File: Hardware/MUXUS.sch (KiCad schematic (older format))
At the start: 3 parts

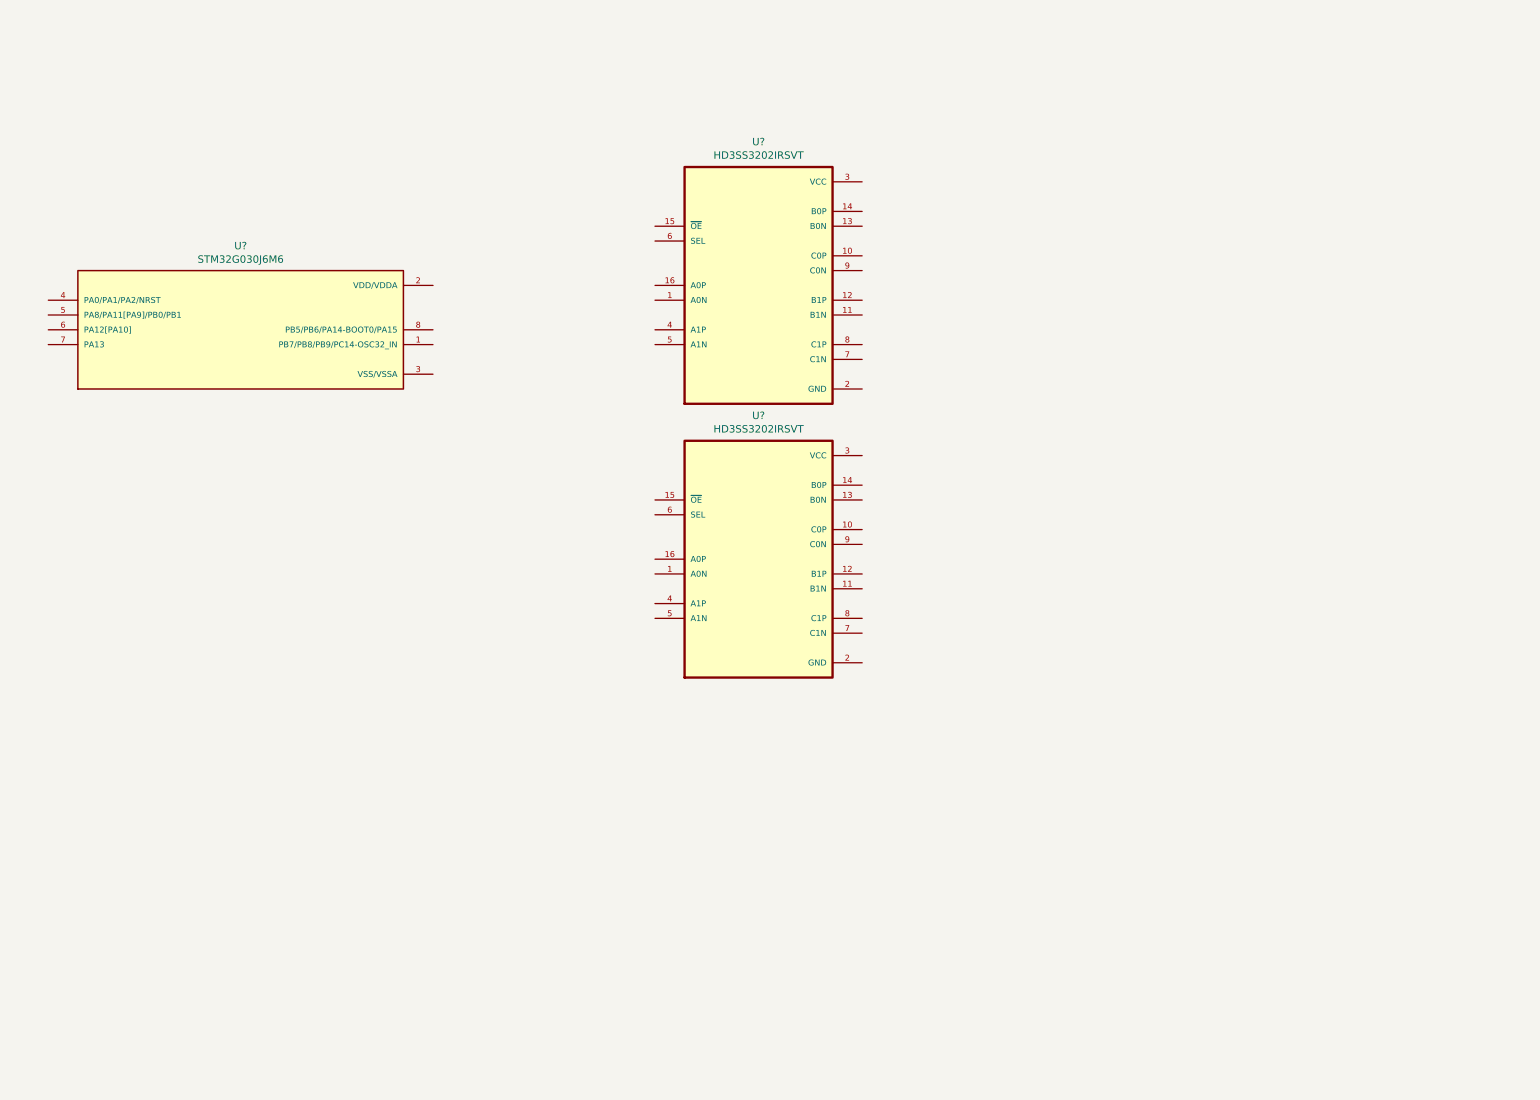
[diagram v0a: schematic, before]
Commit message: Checkpoint
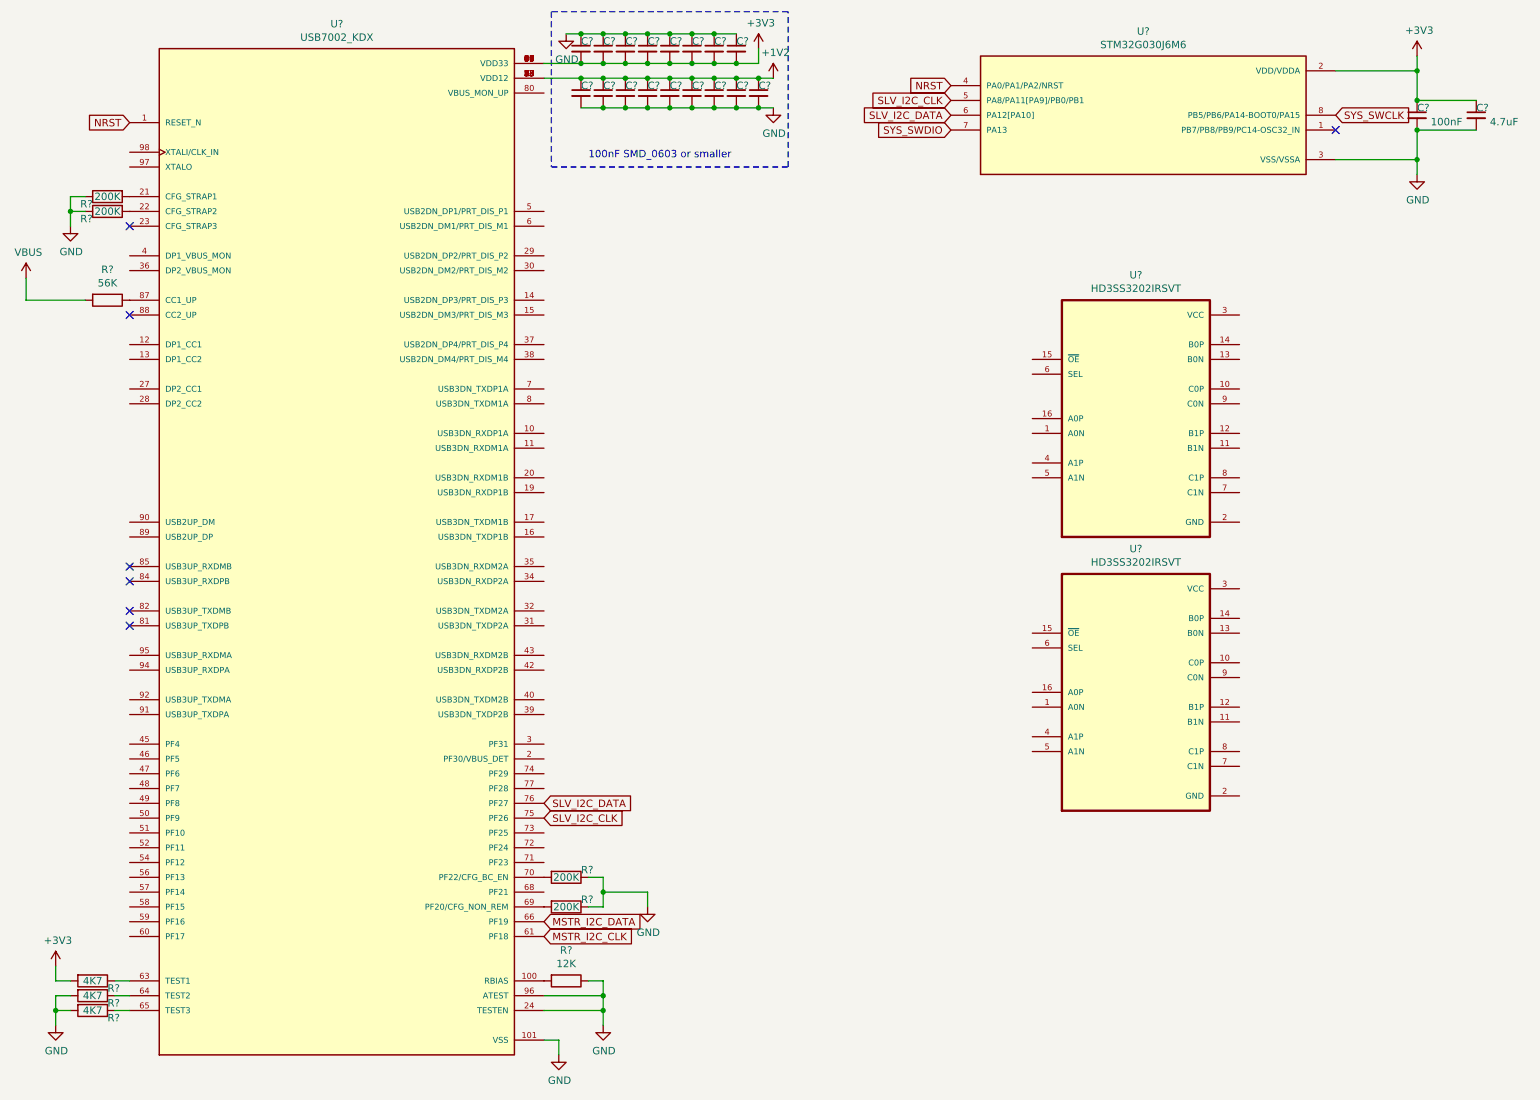
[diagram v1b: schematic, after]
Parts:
- added C? (x18): 100nF, symbol Device:C_Small
- added C?: 4.7uF, symbol Device:C_Small
- added R?: 12K, symbol Device:R
- added R? (x3): 4K7, symbol Device:R
- added R? (x4): 200K, symbol Device:R
- added R?: 56K, symbol Device:R
- added U?: USB7002_KDX, QFN40P1200X1200X90-101N, symbol USB7002_KDX:USB7002_KDX
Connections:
- net +3V3: now reaches U?.2 (VDD/VDDA)
- net +3V3: now also C?.1, C?.1, C?.2, C?.2, C?.2, C?.2, C?.2, C?.2, C?.2, C?.2, R?.2, U?.26 (VDD33), U?.44 (VDD33), U?.53 (VDD33), U?.62 (VDD33), U?.67 (VDD33), U?.79 (VDD33), U?.86 (VDD33), U?.99 (VDD33)
- net GND: now reaches U?.3 (VSS/VSSA)
- net GND: now also C?.1, C?.1, C?.1, C?.1, C?.1, C?.1, C?.1, C?.1, C?.2, C?.2, C?.2, C?.2, C?.2, C?.2, C?.2, C?.2, C?.2, C?.2, C?.2, R?.1, R?.1, R?.1, R?.1, R?.1, R?.2, R?.2, U?.101 (VSS), U?.24 (TESTEN), U?.96 (ATEST)
- net NRST: now reaches U?.4 (PA0/PA1/PA2/NRST)
- net NRST: now also U?.1 (RESET_N)
- net SLV_I2C_CLK: now reaches U?.5 (PA8/PA11[PA9]/PB0/PB1)
- net SLV_I2C_CLK: now also U?.75 (PF26)
- net SLV_I2C_DATA: now reaches U?.6 (PA12[PA10])
- net SLV_I2C_DATA: now also U?.76 (PF27)
- net SYS_SWDIO: now reaches U?.7 (PA13)
- net SYS_SWCLK: now reaches U?.8 (PB5/PB6/PA14-BOOT0/PA15)
- new net: R?.2, U?.100 (RBIAS)
- new net: R?.2, U?.21 (CFG_STRAP1)
- new net: R?.2, U?.22 (CFG_STRAP2)
- new net: R?.1, U?.63 (TEST1)
- new net: R?.1, U?.64 (TEST2)
- new net: R?.1, U?.65 (TEST3)
- new net: R?.2, U?.69 (PF20/CFG_NON_REM)
- new net: R?.2, U?.70 (PF22/CFG_BC_EN)
- new net: R?.1, U?.87 (CC1_UP)
- new net +1V2: C?.1, C?.1, C?.1, C?.1, C?.1, C?.1, C?.1, C?.1, C?.1, U?.18 (VDD12), U?.25 (VDD12), U?.33 (VDD12), U?.41 (VDD12), U?.55 (VDD12), U?.78 (VDD12), U?.83 (VDD12), U?.9 (VDD12), U?.93 (VDD12)
- new net MSTR_I2C_CLK: U?.61 (PF18)
- new net MSTR_I2C_DATA: U?.66 (PF19)
- new net VBUS: R?.2
- no-connect marks 0 -> 7
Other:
- note added: "100nF SMD_0603 or smaller"
- moved on the sheet: U?

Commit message: Checkpoint
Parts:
- removed C? (x18): 100nF, symbol Device:C_Small
- removed C?: 4.7uF, symbol Device:C_Small
- removed R?: 12K, symbol Device:R
- removed R? (x3): 4K7, symbol Device:R
- removed R? (x4): 200K, symbol Device:R
- removed R?: 56K, symbol Device:R
- removed U? (x2): HD3SS3202IRSVT, QFN40P180X260X55-16N_HD3SS3202IRSVT, symbol HD3SS3202IRSVT:HD3SS3202IRSVT
- removed U?: STM32G030J6M6, SOIC127P600X175-8N, symbol STM32G030J6M6:STM32G030J6M6
- removed U?: USB7002_KDX, QFN40P1200X1200X90-101N, symbol USB7002_KDX:USB7002_KDX
- added C? (x11): 100nF, Capacitor_SMD:C_0805_2012Metric, symbol Device:C_Small
- added C? (x5): 4.7uF, symbol Device:C_Small
- added C?: 87pF, symbol Device:C
- added C? (x14): 100nF, Capacitor_SMD:C_0805_2012Metric, symbol Device:C
- added C?: 1uF, symbol Device:C_Small
- added C? (x2): 22uF, symbol Device:C
- added C?: 1uF, symbol Device:C
- added C? (x2): 14pF, symbol Device:C
- added C? (x3): 120uF, Capacitor_SMD:C_0805_2012Metric, symbol Device:C
- added D? (x4): AMBER, LED_SMD:LED_1206_3216Metric, symbol Device:LED
- added D? (x4): GREEN, LED_SMD:LED_1206_3216Metric, symbol Device:LED
- added D?: B540C-13-F, Diode_SMD:D_SMC, symbol Device:D_Schottky
- added D? (x4): LED, symbol Device:LED
- added F?: 500mA, Fuse:Fuse_1206_3216Metric, symbol Device:Polyfuse
- added J? (x3): USB_B, 67068-9000:67068-9000, symbol Connector:USB_B
- added J? (x3): USB_A, 67643-0910:67643-0910, symbol Connector:USB_A
- added J?: USB_C_Receptacle_USB2.0, DX07S016JA1R1500:DX07S016JA1R1500, symbol Connector:USB_C_Receptacle_USB2.0
- added J?: STDC14, symbol Connector_Generic:Conn_02x07_Odd_Even
- added L?: SRP6530A-6R8M, SRP6530A-6R8M:SRP6530A-6R8M, symbol Device:L
- added R? (x4): 10K, Resistor_SMD:R_1206_3216Metric, symbol Device:R
- added R?: 15.1K, symbol Device:R
- added R? (x7): 330R, symbol Device:R
- added R?: 31.6K, symbol Device:R_Small
- added R?: 10K, Resistor_SMD:R_1206_3216Metric, symbol Device:R_Small
- added R? (x3): 1K, symbol Device:R
- added R? (x12): 100R, symbol Device:R
- added R?: 12K, symbol Device:R
- added SW?: USER, symbol Switch:SW_Push
- added SW?: RESET, symbol Switch:SW_Push
- added U?: STM32G431K8T6, STM32G431K8T6:STM32G431K8T6, symbol STM32G431K8T6:STM32G431K8T6
- added U?: AOZ1212AI, Package_SO:SO-8_3.9x4.9mm_P1.27mm, symbol AOZ1212AI:AOZ1212AI
- added U?: TS3USBCA420RSVR, symbol TS3USBCA420RSVR:TS3USBCA420RSVR
- added U? (x6): USBLC6-2SC6, Package_TO_SOT_SMD:SOT-23-6, symbol Power_Protection:USBLC6-2SC6
- added U? (x3): AP2151W, Package_TO_SOT_SMD:SOT-23-5, symbol AP2151W:AP2151W
- added U?: USB2504A-JT, Package_QFP:LQFP-64_10x10mm_P0.5mm, symbol USB2504A-JT:USB2504A-JT
- added U?: USBLC6-4SC6, Package_TO_SOT_SMD:SOT-23-6, symbol Power_Protection:USBLC6-4SC6
- added Y?: ATS240C, symbol Device:Crystal
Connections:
- net +3V3: now also C?.1, C?.1, C?.1, C?.1, C?.1, C?.1, C?.2, C?.2, C?.2, C?.2, C?.2, C?.2, J?.3 (Pin_3), L?.2, R?.1, R?.1, R?.1, R?.1, R?.1, R?.1, R?.1, R?.1, R?.1, R?.2, R?.2, R?.2, R?.2, R?.2, R?.2, R?.2, R?.2, R?.2, R?.2, U?.1 (VCC), U?.1 (VDD), U?.1 (VDDA33), U?.12 (I2C_EN), U?.13 (VDDA33), U?.15 (VDDA/VREF+), U?.17 (VDD), U?.23 (PRTPWR_POL), U?.28 (VDD33), U?.51 (SELF_PWR), U?.61 (VDDA33PLL), U?.62 (ATEST/REG_EN), U?.7 (VDDA33)
- net GND: now also C?.1, C?.1, C?.1, C?.1, C?.1, C?.1, C?.1, C?.1, C?.1, C?.1, C?.1, C?.1, C?.1, C?.1, C?.1, C?.1, C?.1, C?.1, C?.1, C?.1, C?.1, C?.1, C?.1, C?.2, C?.2, C?.2, C?.2, C?.2, C?.2, C?.2, C?.2, C?.2, C?.2, C?.2, C?.2, C?.2, C?.2, C?.2, C?.2, D?.2 (A), J?.4 (GND), J?.4 (GND), J?.4 (GND), J?.4 (GND), J?.4 (GND), J?.4 (GND), J?.5 (Pin_5), J?.7 (Pin_7), J?.A1 (GND), J?.A12 (GND), J?.B1 (GND), J?.B12 (GND), R?.1, R?.1, R?.1, R?.1, R?.2, R?.2, R?.2, R?.2, R?.2, R?.2, SW?.2, SW?.2, U?.10 (VSS), U?.14 (VSSA), U?.16 (VSS), U?.16 (VSS), U?.2 (GND), U?.2 (GND), U?.2 (GND), U?.2 (GND), U?.2 (GND), U?.2 (GND), U?.2 (GND), U?.2 (GND), U?.2 (GND), U?.2 (GND), U?.29 (VSS), U?.3 (GND), U?.31 (TEST0), U?.32 (VSS), U?.36 (CFG_SEL0), U?.4 (OEn), U?.4 (VSS), U?.41 (VSS), U?.47 (CLKIN_EN), U?.48 (TEST1), U?.50 (CFG_SEL1), U?.53 (VSS), U?.55 (VSS), U?.59 (CFG_SEL2), U?.64 (VSS), U?.9 (GND)
- net NRST: now also C?.2, J?.12 (Pin_12), R?.1, SW?.1, U?.4 (PG10-NRST)
- net VBUS: now also C?.2, C?.2, C?.2, U?.5 (IN), U?.5 (IN), U?.5 (IN)
- new net: C?.2, D?.1 (K), L?.1, U?.1 (LX)
- new net: C?.1, U?.2 (BST)
- new net: R?.1, R?.2, U?.4 (FB)
- new net: R?.2, U?.5 (COMP)
- new net: C?.2, F?.1, U?.6 (EN), U?.7 (VIN)
- new net: C?.2, U?.8 (VBIAS)
- new net: C?.2, R?.1
- new net: C?.2, J?.S1 (SHIELD), R?.2
- new net: C?.1, J?.5 (Shield), R?.1 (x3)
- new net: C?.1, C?.1, J?.1 (VBUS), U?.1 (OUT), U?.5 (VBUS) (x3)
- new net: C?.2, J?.5 (Shield), R?.2 (x3)
- new net: C?.1, U?.57 (XTAL2), Y?.1
- new net: C?.2, U?.58 (XTAL1/CLKIN), Y?.2
- new net: D?.1 (K), U?.19 (AM4/LED_EN)
- new net: D?.1 (K), U?.20 (GR4/PRT_DIS1)
- new net: D?.1 (K), U?.21 (AM3)
- new net: D?.1 (K), U?.22 (GR3/PRT_DIS0)
- new net: D?.1 (K), U?.24 (AM2/MTT_EN)
- new net: D?.1 (K), U?.25 (GR2/NON_REM1)
- new net: D?.1 (K), U?.26 (AM1/GANG_EN)
- new net: D?.1 (K), U?.27 (GR1/NON_REM0)
- new net: C?.2, C?.2, C?.2, C?.2, U?.30 (VDD18), U?.42 (VDD18), U?.54 (VDD18), U?.60 (VDDA18PLL)
- new net: R?.1, U?.63 (RBIAS)
- new net: D?.2 (A), R?.1 (x8)
- new net: D?.2 (A), R?.2 (x4)
- new net BOOT0: R?.1, U?.31 (PB8-BOOT0)
- new net CC1: J?.A5 (CC1), U?.19 (PA9), U?.29 (PB6), U?.4 (I/O3)
- new net CC2: J?.B5 (CC2), U?.20 (PA10), U?.27 (PB4), U?.6 (I/O4)
- new net DFP1_D+: U?.22 (PA12), U?.6 (USBDP1)
- new net DFP1_D-: U?.21 (PA11), U?.5 (USBDN1)
- new net DFP2_CONN_D+: J?.3 (D+), U?.3 (I/O2)
- new net DFP2_CONN_D-: J?.2 (D-), U?.1 (I/O1)
- new net DFP2_D+: U?.4 (I/O2), U?.8 (USBDP2)
- new net DFP2_D-: U?.6 (I/O1), U?.9 (USBDN2)
- new net DFP2_EN: U?.4 (EN), U?.43 (PRTPWR2)
- new net DFP2_OCSn: U?.3 (~FLG), U?.44 (OCS2_N)
- new net DFP3_CONN_D+: J?.3 (D+), U?.3 (I/O2)
- new net DFP3_CONN_D-: J?.2 (D-), U?.1 (I/O1)
- new net DFP3_D+: U?.12 (USBDP3), U?.4 (I/O2)
- new net DFP3_D-: U?.11 (USBDN3), U?.6 (I/O1)
- new net DFP3_EN: U?.39 (PRTPWR3), U?.4 (EN)
- new net DFP3_OCSn: U?.3 (~FLG), U?.40 (OCS3_N)
- new net DFP4_CONN_D+: J?.3 (D+), U?.3 (I/O2)
- new net DFP4_CONN_D-: J?.2 (D-), U?.1 (I/O1)
- new net DFP4_D+: U?.14 (USBDP4), U?.4 (I/O2)
- new net DFP4_D-: U?.15 (USBDN4), U?.6 (I/O1)
- new net DFP4_EN: U?.37 (PRTPWR4), U?.4 (EN)
- new net DFP4_OCSn: U?.3 (~FLG), U?.38 (OCS4_N)
- new net HUB_RESET: R?.2, U?.13 (PB0), U?.49 (RESET_N)
- new net I2C1_SCL: U?.25 (PA15), U?.35 (SCL/SMBCLK), U?.5 (SEL1/SCL)
- new net I2C1_SDA: R?.2, U?.30 (PB7), U?.34 (SDA/SMBDATA), U?.6 (SEL0/SDA)
- new net I2C1_SMBA: R?.2, U?.28 (PB5)
- new net IFP_D+: U?.11 (SBU1), U?.2 (USBDP0)
- new net IFP_D-: U?.10 (SBU2), U?.3 (USBDN0)
- new net IFP_VBUS: R?.2, U?.12 (PA7), U?.52 (VBUS_DET)
- new net LPUART1_RX: J?.13 (Pin_13), U?.8 (PA3)
- new net LPUART1_TX: J?.14 (Pin_14), U?.7 (PA2)
- new net SWCLK: J?.6 (Pin_6), U?.24 (PA14)
- new net SWDIO: J?.4 (Pin_4), U?.23 (PA13)
- new net SWO: J?.8 (Pin_8), U?.26 (PB3)
- new net UFP1_D+: J?.A6 (D+), J?.B6 (D+), U?.3 (I/O2), U?.7 (LnBp)
- new net UFP1_D-: J?.A7 (D-), J?.B7 (D-), U?.1 (I/O1), U?.8 (LnBn)
- new net UFP1_VBUS: F?.2, J?.A4 (VBUS), J?.A9 (VBUS), J?.B4 (VBUS), J?.B9 (VBUS), U?.5 (VBUS)
- new net UFP2_CONN_D+: J?.3 (D+), U?.1 (I/O1)
- new net UFP2_CONN_D-: J?.2 (D-), U?.3 (I/O2)
- new net UFP2_D+: U?.2 (MIC_GND1/Ln1), U?.6 (I/O1)
- new net UFP2_D-: U?.3 (MIC_GND2/Ln2), U?.4 (I/O2)
- new net UFP2_VBUS: J?.1 (VBUS), U?.5 (VBUS), U?.9 (PA4)
- new net UFP3_CONN_D+: J?.3 (D+), U?.1 (I/O1)
- new net UFP3_CONN_D-: J?.2 (D-), U?.3 (I/O2)
- new net UFP3_D+: U?.14 (LnCp), U?.6 (I/O1)
- new net UFP3_D-: U?.13 (LnCn), U?.4 (I/O2)
- new net UFP3_VBUS: J?.1 (VBUS), U?.10 (PA5), U?.5 (VBUS)
- new net UFP4_CONN_D+: J?.3 (D+), U?.1 (I/O1)
- new net UFP4_CONN_D-: J?.2 (D-), U?.3 (I/O2)
- new net UFP4_D+: U?.16 (LnAp), U?.6 (I/O1)
- new net UFP4_D-: U?.15 (LnAn), U?.4 (I/O2)
- new net UFP4_VBUS: J?.1 (VBUS), U?.11 (PA6), U?.5 (VBUS)
- new net UI_BUTTON: C?.2, R?.1, SW?.1, U?.18 (PA8)
- new net UI_LED1: D?.1 (K), U?.2 (PF0-OSC_IN)
- new net UI_LED2: D?.1 (K), U?.3 (PF1-OSC_OUT)
- new net UI_LED3: D?.1 (K), U?.5 (PA0)
- new net UI_LED4: D?.1 (K), U?.6 (PA1)
- no-connect marks 7 -> 9
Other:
- note added: "create footprint"
- note removed: "100nF SMD_0603 or smaller"
